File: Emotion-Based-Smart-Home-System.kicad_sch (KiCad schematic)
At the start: 10 parts, among them J1 Barrel_Jack, Q1 BC107, U1 HC-SR04, U3 JTE0624D03

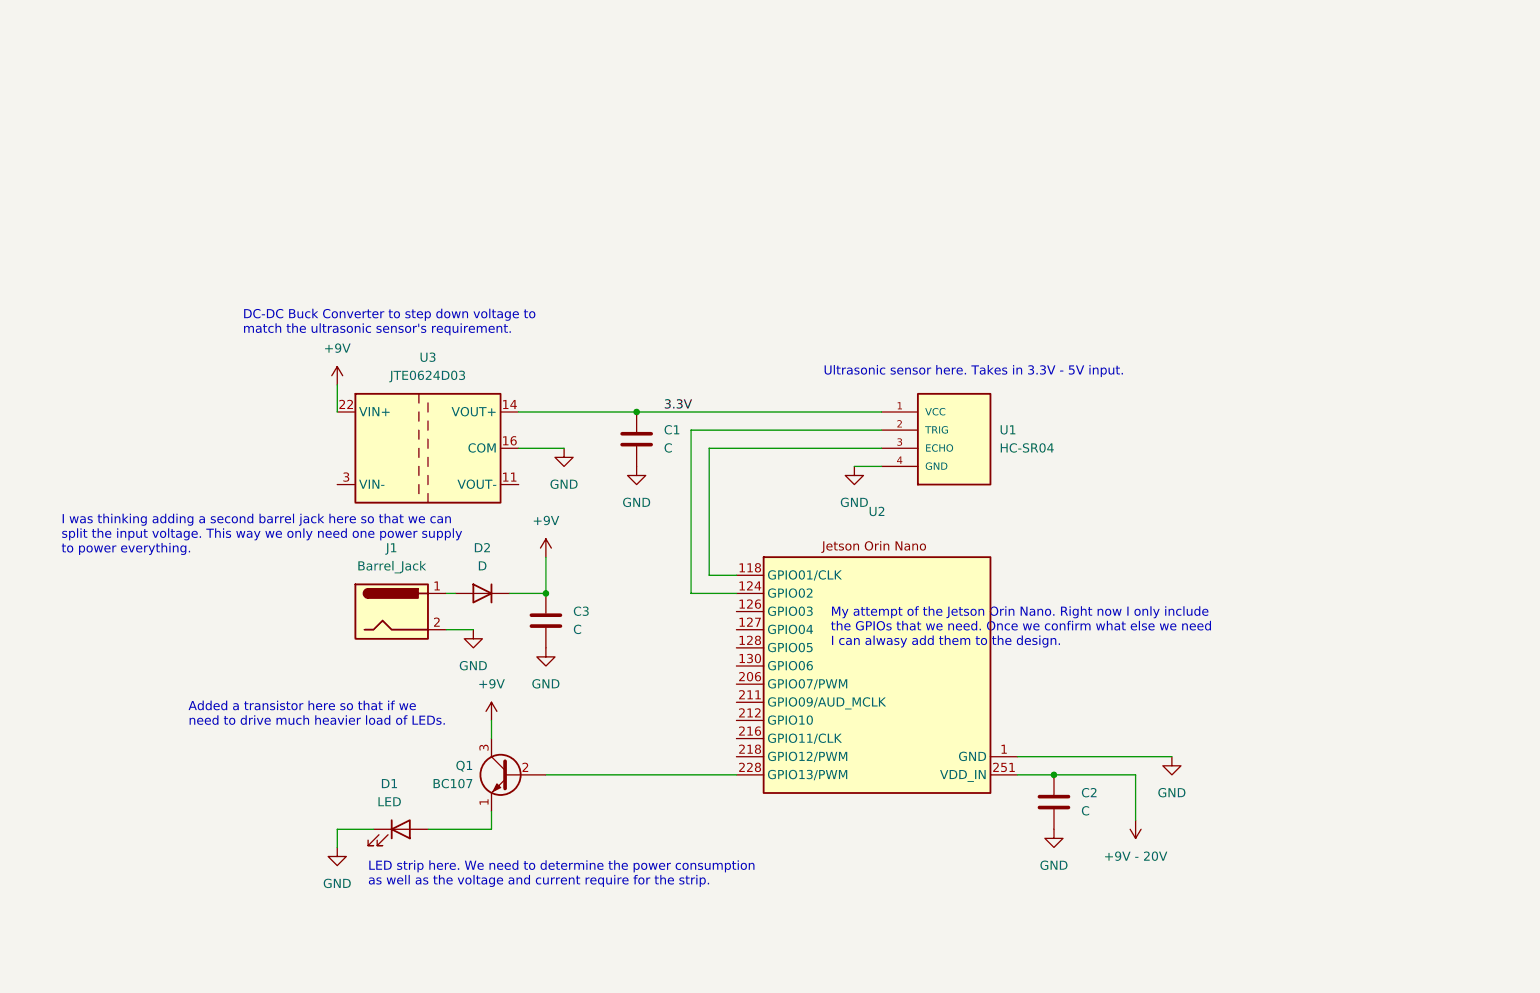
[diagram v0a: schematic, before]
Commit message: Current updated schematic
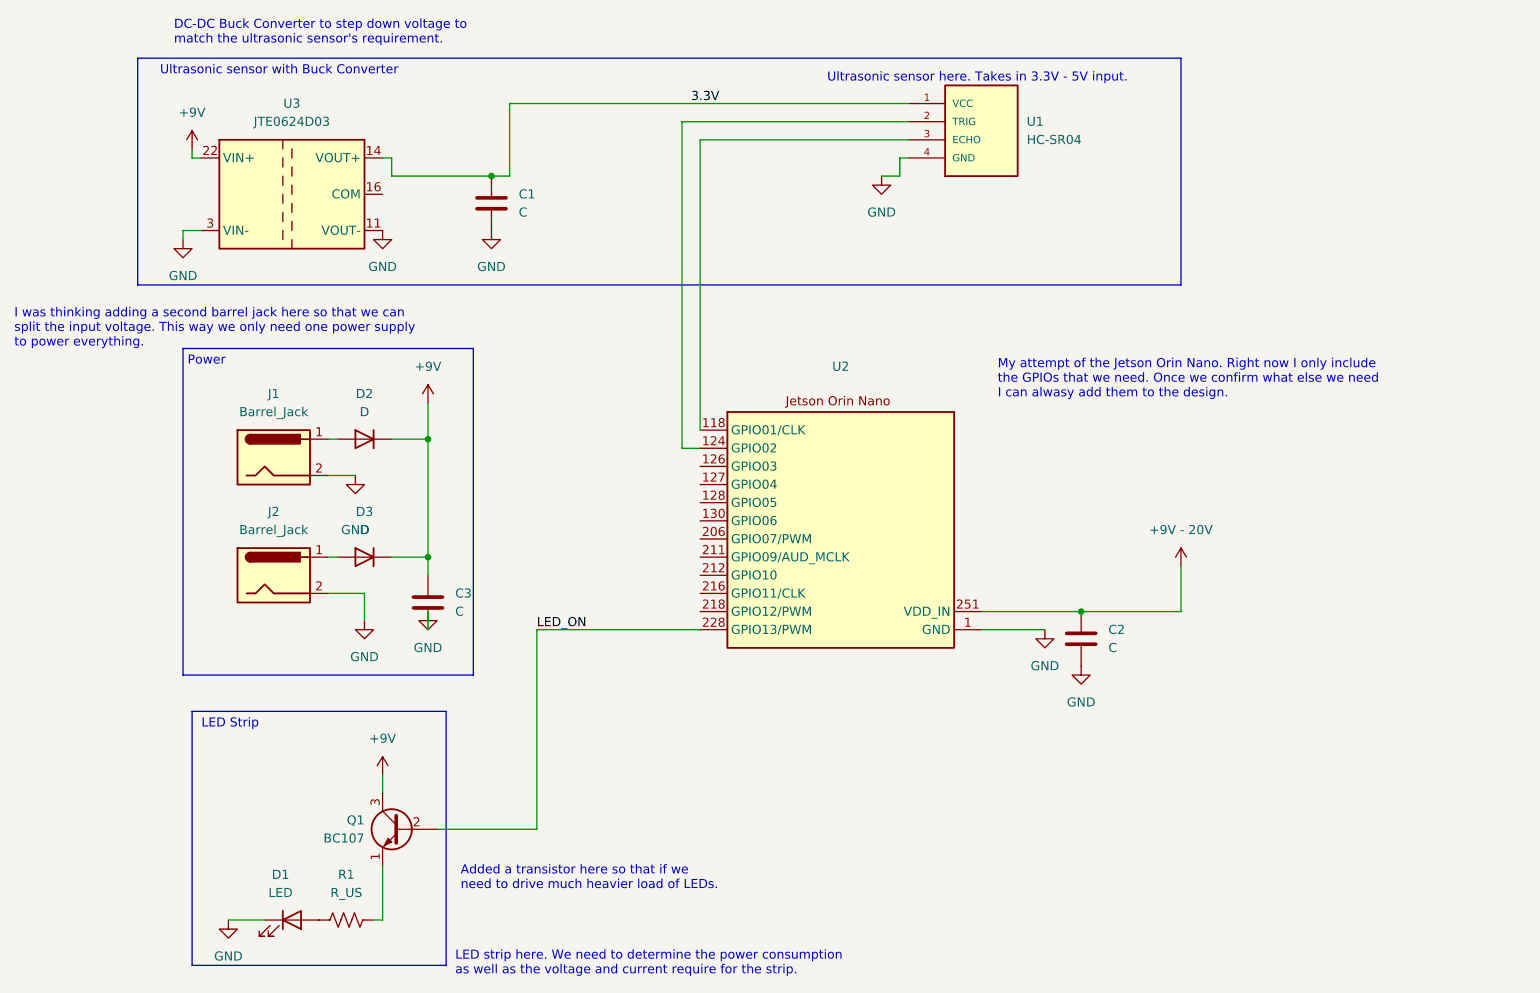
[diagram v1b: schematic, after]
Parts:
- added D3: D, symbol Device:D
- added J2: Barrel_Jack, symbol Connector:Barrel_Jack
- added R1: R_US, symbol Device:R_US
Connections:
- net +9V: now also D3.1 (K)
- net GND: now also U3.11 (VOUT-), U3.2 (VIN-), U3.3 (VIN-), J2.2; no longer U3.16 (COM), U3.9 (COM)
- net at Q1.1 (E): now also R1.2; no longer D1.2 (A)
- net LED_ON: now reaches Q1.2 (B), U2.228 (GPIO13/PWM)
- new net: D3.2 (A), J2.1
- new net: U3.16 (COM), U3.9 (COM)
- new net: D1.2 (A), R1.1
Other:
- note added: "LED Strip"
- note added: "Power"
- note added: "Ultrasonic sensor with Buck Converter"
- title: Emotion-Based-Smart-Home-System  -> Emotion-Adaptive-Smart-Home
- moved on the sheet: C1, C3, D1, D2, J1, Q1, U1, U2, U3
